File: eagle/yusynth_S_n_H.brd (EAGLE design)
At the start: 100 x 80 mm, 43 parts, among them IC1 TL074P, IC2 TL071P, Q1 BF245, T1 2N3904

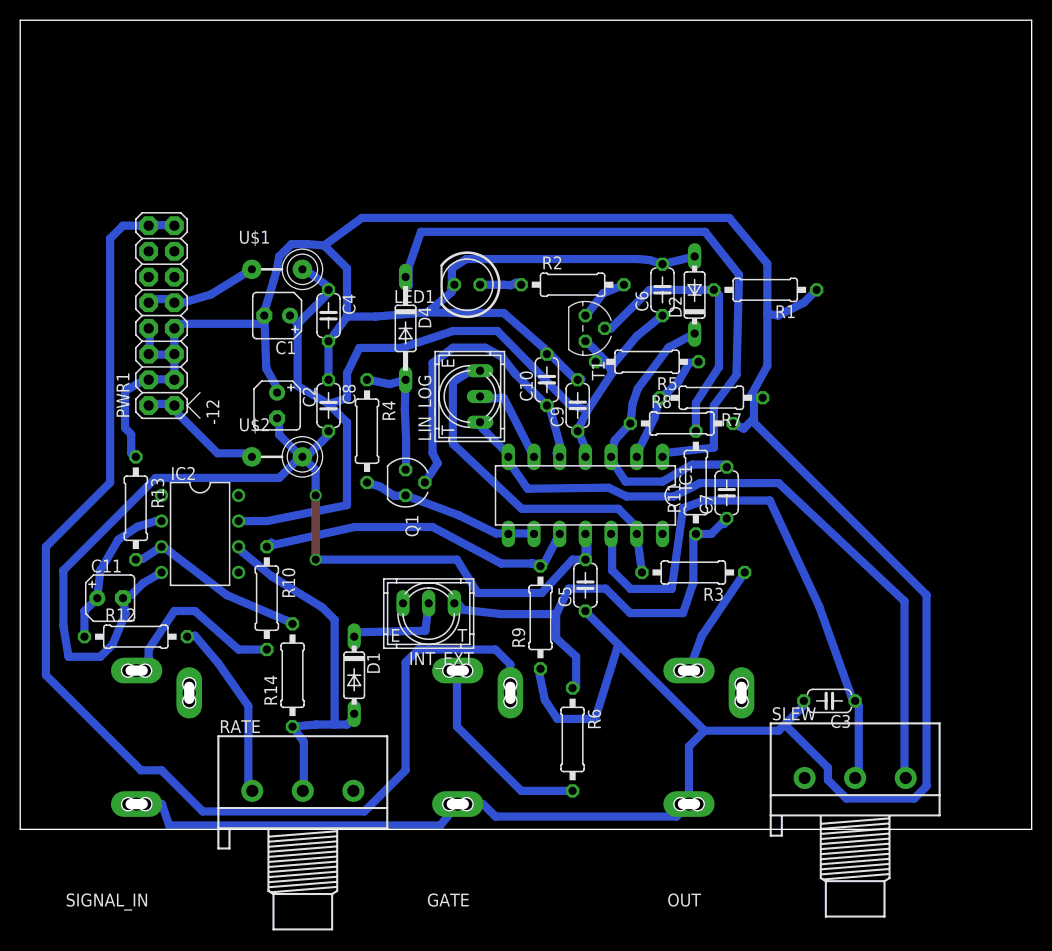
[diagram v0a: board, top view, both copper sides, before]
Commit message: cutout
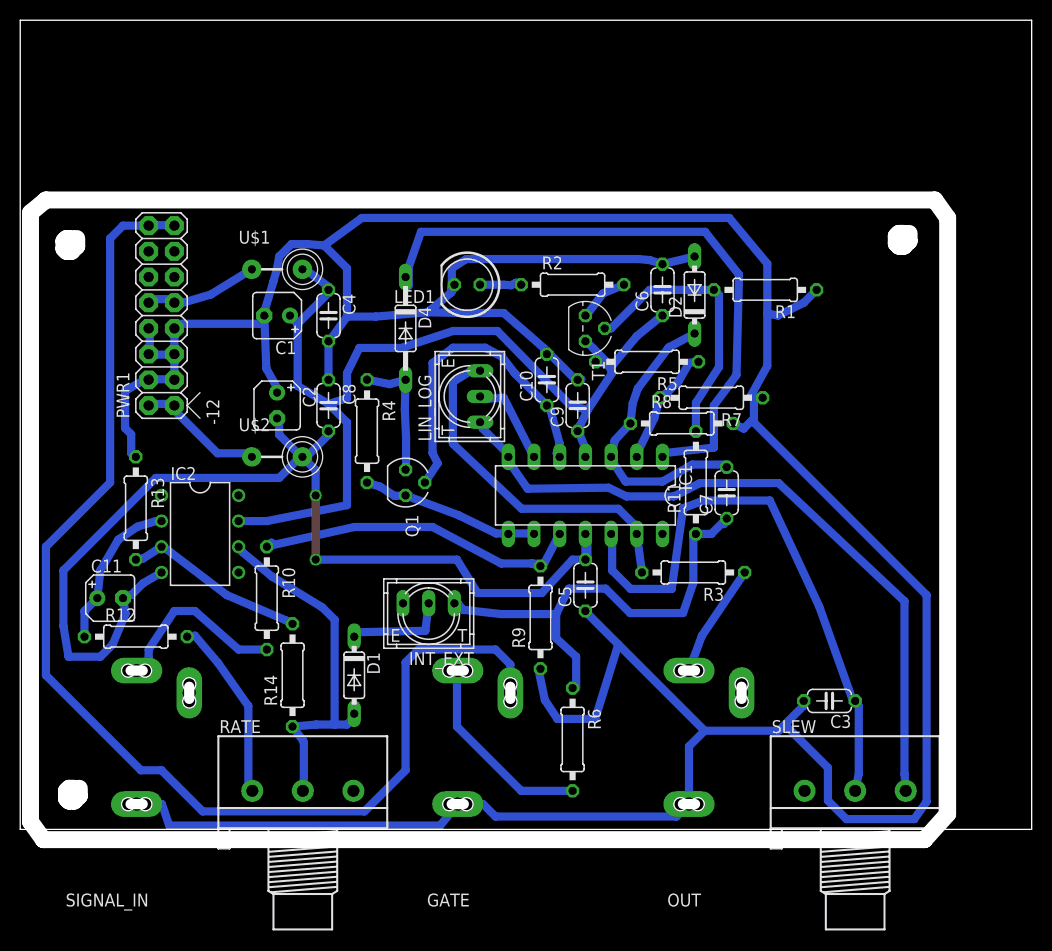
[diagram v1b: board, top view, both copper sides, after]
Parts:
- moved SLEW 1.27 mm to (82.5, 3.81)
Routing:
- net GND: track 369.5 -> 373.4 mm
- net N$19: track 68.2 -> 69.5 mm
- net N$13: track 56.5 -> 57.7 mm
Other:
- board size 100 x 80 mm -> 100 x 81 mm
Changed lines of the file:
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@@
 <layer number="44" name="Drills" color="7" fill="1" visible="no" active="yes"/>
 <layer number="45" name="Holes" color="7" fill="1" visible="no" active="yes"/>
-<layer number="46" name="Milling" color="3" fill="1" visible="no" active="yes"/>
+<layer number="46" name="Milling" color="3" fill="1" visible="yes" active="yes"/>
 <layer number="47" name="Measures" color="7" fill="1" visible="no" active="yes"/>
 <layer number="48" name="Document" color="7" fill="1" visible="yes" active="yes"/>
@@
 <wire x1="100" y1="80" x2="0" y2="80" width="0" layer="20"/>
 <wire x1="0" y1="80" x2="0" y2="0" width="0" layer="20"/>
+<wire x1="2.286" y1="-1.016" x2="1.016" y2="0.762" width="1.6764" layer="46"/>
+<wire x1="1.016" y1="0.762" x2="1.016" y2="60.96" width="1.6764" layer="46"/>
+<wire x1="1.016" y1="60.96" x2="2.54" y2="62.23" width="1.6764" layer="46"/>
+<wire x1="2.54" y1="62.23" x2="90.424" y2="62.23" width="1.6764" layer="46"/>
+<wire x1="90.424" y1="62.23" x2="91.694" y2="60.452" width="1.6764" layer="46"/>
+<wire x1="91.694" y1="60.452" x2="91.694" y2="1.524" width="1.6764" layer="46"/>
+<wire x1="91.694" y1="1.524" x2="89.408" y2="-1.016" width="1.6764" layer="46"/>
+<wire x1="89.408" y1="-1.016" x2="2.286" y2="-1.016" width="1.6764" layer="46"/>
+<wire x1="5.08" y1="58.42" x2="4.572" y2="58.42" width="1.6764" layer="46"/>
+<wire x1="4.572" y1="58.42" x2="4.318" y2="58.166" width="1.6764" layer="46"/>
+<wire x1="4.318" y1="58.166" x2="4.318" y2="57.404" width="1.6764" layer="46"/>
+<wire x1="4.318" y1="57.404" x2="4.572" y2="57.15" width="1.6764" layer="46"/>
+<wire x1="4.572" y1="57.15" x2="5.08" y2="57.15" width="1.6764" layer="46"/>
+<wire x1="5.08" y1="57.15" x2="5.588" y2="57.658" width="1.6764" layer="46"/>
+<wire x1="5.588" y1="57.658" x2="5.588" y2="58.42" width="1.6764" layer="46"/>
+<wire x1="87.376" y1="58.928" x2="86.868" y2="58.928" width="1.6764" layer="46"/>
+<wire x1="86.868" y1="58.928" x2="86.614" y2="58.674" width="1.6764" layer="46"/>
+<wire x1="86.614" y1="58.674" x2="86.614" y2="57.912" width="1.6764" layer="46"/>
+<wire x1="86.614" y1="57.912" x2="86.868" y2="57.658" width="1.6764" layer="46"/>
+<wire x1="86.868" y1="57.658" x2="87.376" y2="57.658" width="1.6764" layer="46"/>
+<wire x1="87.376" y1="57.658" x2="87.884" y2="58.166" width="1.6764" layer="46"/>
+<wire x1="87.884" y1="58.166" x2="87.884" y2="58.928" width="1.6764" layer="46"/>
+<wire x1="5.334" y1="4.064" x2="4.826" y2="4.064" width="1.6764" layer="46"/>
+<wire x1="4.826" y1="4.064" x2="4.572" y2="3.81" width="1.6764" layer="46"/>
+<wire x1="4.572" y1="3.81" x2="4.572" y2="3.048" width="1.6764" layer="46"/>
+<wire x1="4.572" y1="3.048" x2="4.826" y2="2.794" width="1.6764" layer="46"/>
+<wire x1="4.826" y1="2.794" x2="5.334" y2="2.794" width="1.6764" layer="46"/>
+<wire x1="5.334" y1="2.794" x2="5.842" y2="3.302" width="1.6764" layer="46"/>
+<wire x1="5.842" y1="3.302" x2="5.842" y2="4.064" width="1.6764" layer="46"/>
 </plain>
 <attributes>
@@
 <element name="R8" library="rcl" package="0207/10" value="100k" x="65.405" y="40.132"/>
 <element name="R9" library="rcl" package="0207/10" value="100k" x="51.435" y="20.955" rot="R90"/>
-<element name="SLEW" library="pot" package="3RP/1610N" value="1M log" x="82.55" y="5.08"/>
+<element name="SLEW" library="pot" package="3RP/1610N" value="1M log" x="82.55" y="3.81"/>
 <element name="T1" library="transistor" package="TO92" value="2N3904" x="55.88" y="49.53" rot="R270"/>
 <element name="U$1" library="adafruit" package="FB" value="FB" x="25.4" y="55.372"/>
@@
 <wire x1="72.5424" y1="40.64" x2="72.5424" y2="42.672" width="0.8128" layer="16"/>
 <wire x1="89.6112" y1="23.1648" x2="72.5424" y2="40.2336" width="0.8128" layer="16"/>
-<wire x1="89.6112" y1="4.2672" x2="89.6112" y2="23.1648" width="0.8128" layer="16"/>
-<wire x1="88.392" y1="3.048" x2="89.6112" y2="4.2672" width="0.8128" layer="16"/>
-<wire x1="81.6864" y1="3.048" x2="88.392" y2="3.048" width="0.8128" layer="16"/>
-<wire x1="79.8576" y1="4.8768" x2="81.6864" y2="3.048" width="0.8128" layer="16"/>
-<wire x1="79.8576" y1="6.096" x2="79.8576" y2="4.8768" width="0.8128" layer="16"/>
+<wire x1="89.6112" y1="2.7432" x2="89.6112" y2="23.1648" width="0.8128" layer="16"/>
+<wire x1="88.392" y1="1.016" x2="89.6112" y2="2.7432" width="0.8128" layer="16"/>
+<wire x1="81.6864" y1="1.016" x2="88.392" y2="1.016" width="0.8128" layer="16"/>
+<wire x1="79.8576" y1="2.8448" x2="81.6864" y2="1.016" width="0.8128" layer="16"/>
+<wire x1="79.8576" y1="6.096" x2="79.8576" y2="2.8448" width="0.8128" layer="16"/>
 <wire x1="75.5904" y1="10.3632" x2="79.8576" y2="6.096" width="0.8128" layer="16"/>
 <wire x1="72.5424" y1="42.672" x2="73.406" y2="42.672" width="0.8128" layer="16"/>
@@
 <wire x1="82.9056" y1="5.4864" x2="82.9056" y2="12.192" width="0.8128" layer="16"/>
 <wire x1="82.9056" y1="12.192" x2="82.55" y2="12.7" width="0.8128" layer="16"/>
-<wire x1="82.9056" y1="5.4864" x2="82.55" y2="5.08" width="0.8128" layer="16"/>
+<wire x1="82.9056" y1="5.4864" x2="82.55" y2="3.81" width="0.8128" layer="16"/>
 <wire x1="58.5216" y1="25.6032" x2="58.5216" y2="28.6512" width="0.8128" layer="16"/>
 <wire x1="60.3504" y1="23.7744" x2="58.5216" y2="25.6032" width="0.8128" layer="16"/>
@@
 <wire x1="59.944" y1="32.9184" x2="64.6176" y2="32.9184" width="0.8128" layer="16"/>
 <wire x1="48.1584" y1="36.576" x2="50.165" y2="33.6804" width="0.8128" layer="16"/>
-<wire x1="87.4268" y1="5.4864" x2="87.55" y2="5.08" width="0.8128" layer="16"/>
+<wire x1="87.4268" y1="5.4864" x2="87.55" y2="3.81" width="0.8128" layer="16"/>
 <wire x1="48.1584" y1="36.576" x2="48.26" y2="36.83" width="0.8128" layer="16"/>
 </signal>
